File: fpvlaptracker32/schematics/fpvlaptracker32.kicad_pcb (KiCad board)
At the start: 2 copper layers, 49 x 49.9 mm, 27 parts, among them J1 Screw_Terminal_01x03, J2 Serial, SW1 Webupdate, SW2 Prog, SW3 Reset, U1 RX5808, U2 LM1117-3.3, U3 ESP-32_WROOM32

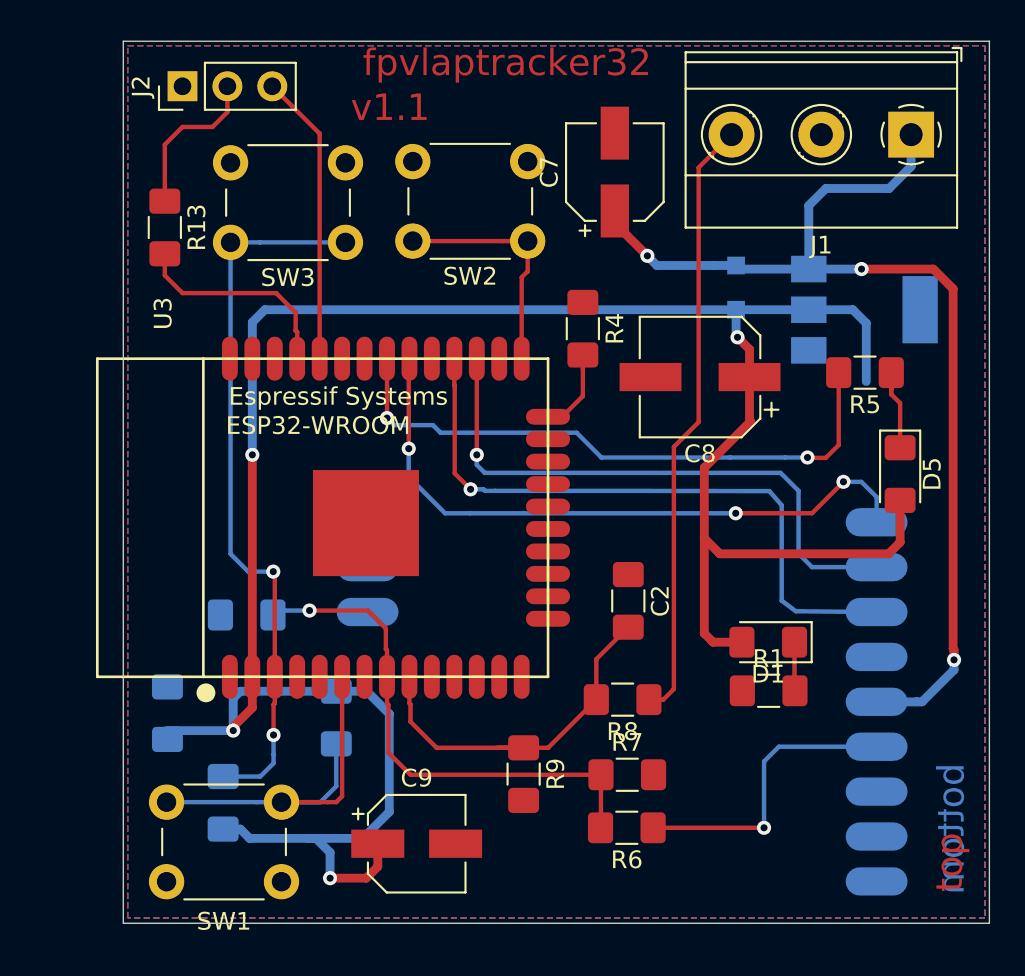
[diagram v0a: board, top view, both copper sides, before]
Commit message: updated rev1.1
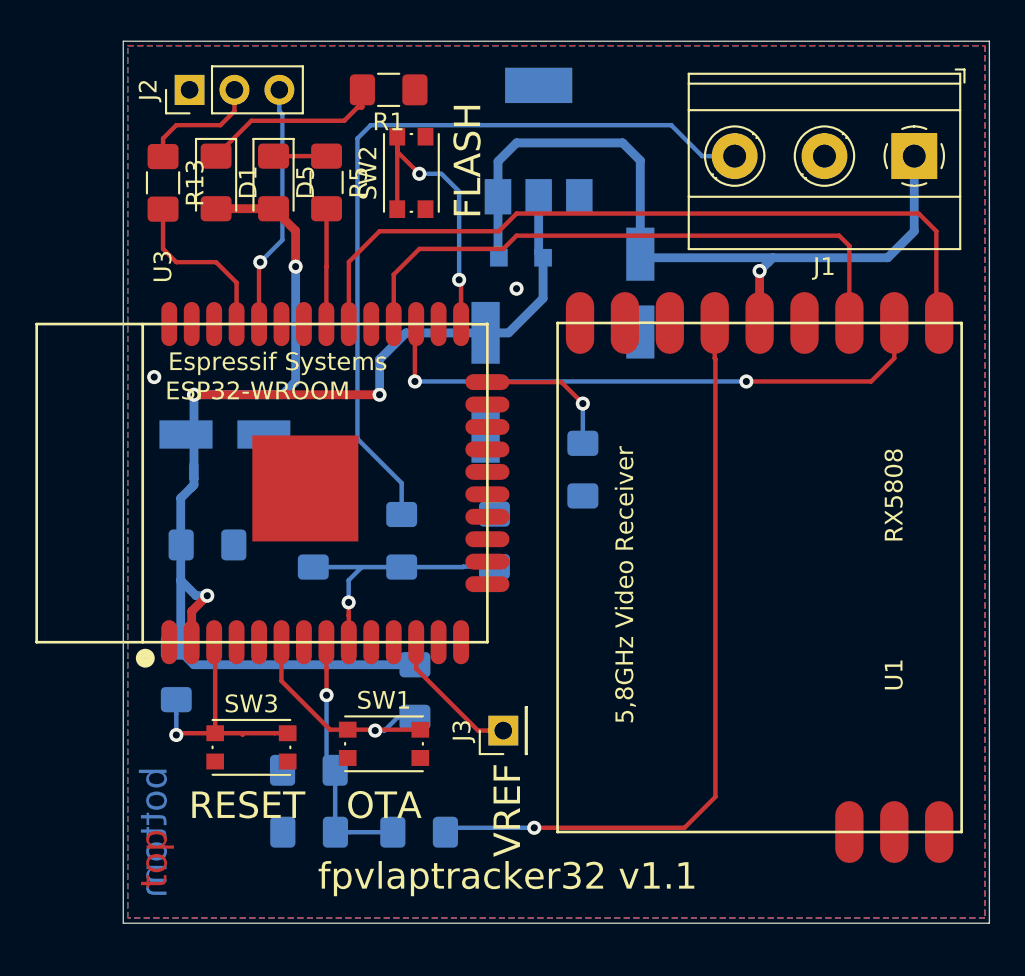
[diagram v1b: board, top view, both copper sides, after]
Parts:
- added J3: Conn_01x01_Female, Connector_PinHeader_2.54mm:PinHeader_1x01_P2.54mm_Vertical, F.Cu at (156.2, 115.2)
- C2, C7, C8, C9, R4, R7, R8: moved to B.Cu
- R5: value 1k -> 100
- R6: value 1k -> 10k; moved to B.Cu
- R9: value 10k -> 1k; moved to B.Cu
- SW1, SW2, SW3: footprint Button_Switch_THT:SW_PUSH_6mm -> Button_Switch_SMD:SW_SPST_KMR2
- U1: moved to F.Cu
- moved D1 40.7 mm to (140.0, 84.2), turned to 270 degrees
- moved R1 40.2 mm to (149.8, 79.0), turned to 180 degrees
- moved D5 39.1 mm to (143.2, 84.2)
- moved R5 32.3 mm to (146.2, 84.2), turned to 270 degrees
- moved SW3 29.1 mm to (142.0, 116.2), turned to 0 degrees
- moved C9 25.6 mm to (140.5, 98.5)
- moved U2 20.8 mm to (158.2, 81.9), turned to 90 degrees
- moved R7 18.3 mm to (145.3, 121.0), turned to 180 degrees
- moved R9 17.8 mm to (145.5, 104.5), turned to 90 degrees
- moved R8 15.4 mm to (150.5, 104.5), turned to 270 degrees
- moved SW1 12.7 mm to (149.5, 116.0)
- moved D4 12.3 mm to (157.2, 88.5), turned to 180 degrees
- moved C8 12.1 mm to (155.2, 95.5), turned to 270 degrees
- moved R6 11.8 mm to (151.5, 121.0)
- moved U1 10.5 mm to (170.8, 105.8), turned to 90 degrees
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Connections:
- U3 pad 12: Net-(U3-Pad12) -> /ADC_REF
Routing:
- net +3V3: track 136.2 -> 83.5 mm
- net /EN: track 41.9 -> 13.6 mm, vias 2 -> 1
- net /LED: track 34.2 -> 6.53 mm, vias 2 -> 0
- net /RSSI: track 16.7 -> 42.9 mm
- net +5V: track 60.0 -> 44.4 mm, vias 3 -> 1
- net /ANALOG_RSSI: track 29.6 -> 14.2 mm
- net /BAT: track 34.4 -> 44.7 mm
- net /WEB_UPDATE: track 22.8 -> 13.8 mm, vias 0 -> 1
- net /ADC_REF: track 0.00 -> 8.13 mm
- net Net-(D1-Pad1): track 2.76 -> 10.4 mm
- net /SPI_DATA: track 36.5 -> 43.6 mm, vias 3 -> 0
- net /ANALOG_BAT: track 21.2 -> 14.8 mm, vias 0 -> 1
- net /IO0: track 13.3 -> 16.9 mm, vias 0 -> 2
- net Net-(R4-Pad2): track 4.78 -> 8.15 mm, vias 0 -> 1
- net /RXD: track 16.5 -> 13.9 mm, vias 0 -> 1
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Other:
- board text added: "+5V GND BAT"
- board text added: "FLASH"
- board text added: "OTA"
- board text added: "RESET"
- board text added: "RX TX GND"
- board text added: "VREF"
- board text added: "fpvlaptracker32 v1.1"
- board text removed: "fpvlaptracker32"
- board text removed: "v1.1"
